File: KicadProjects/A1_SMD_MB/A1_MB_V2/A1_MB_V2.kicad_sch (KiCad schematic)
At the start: 0 parts

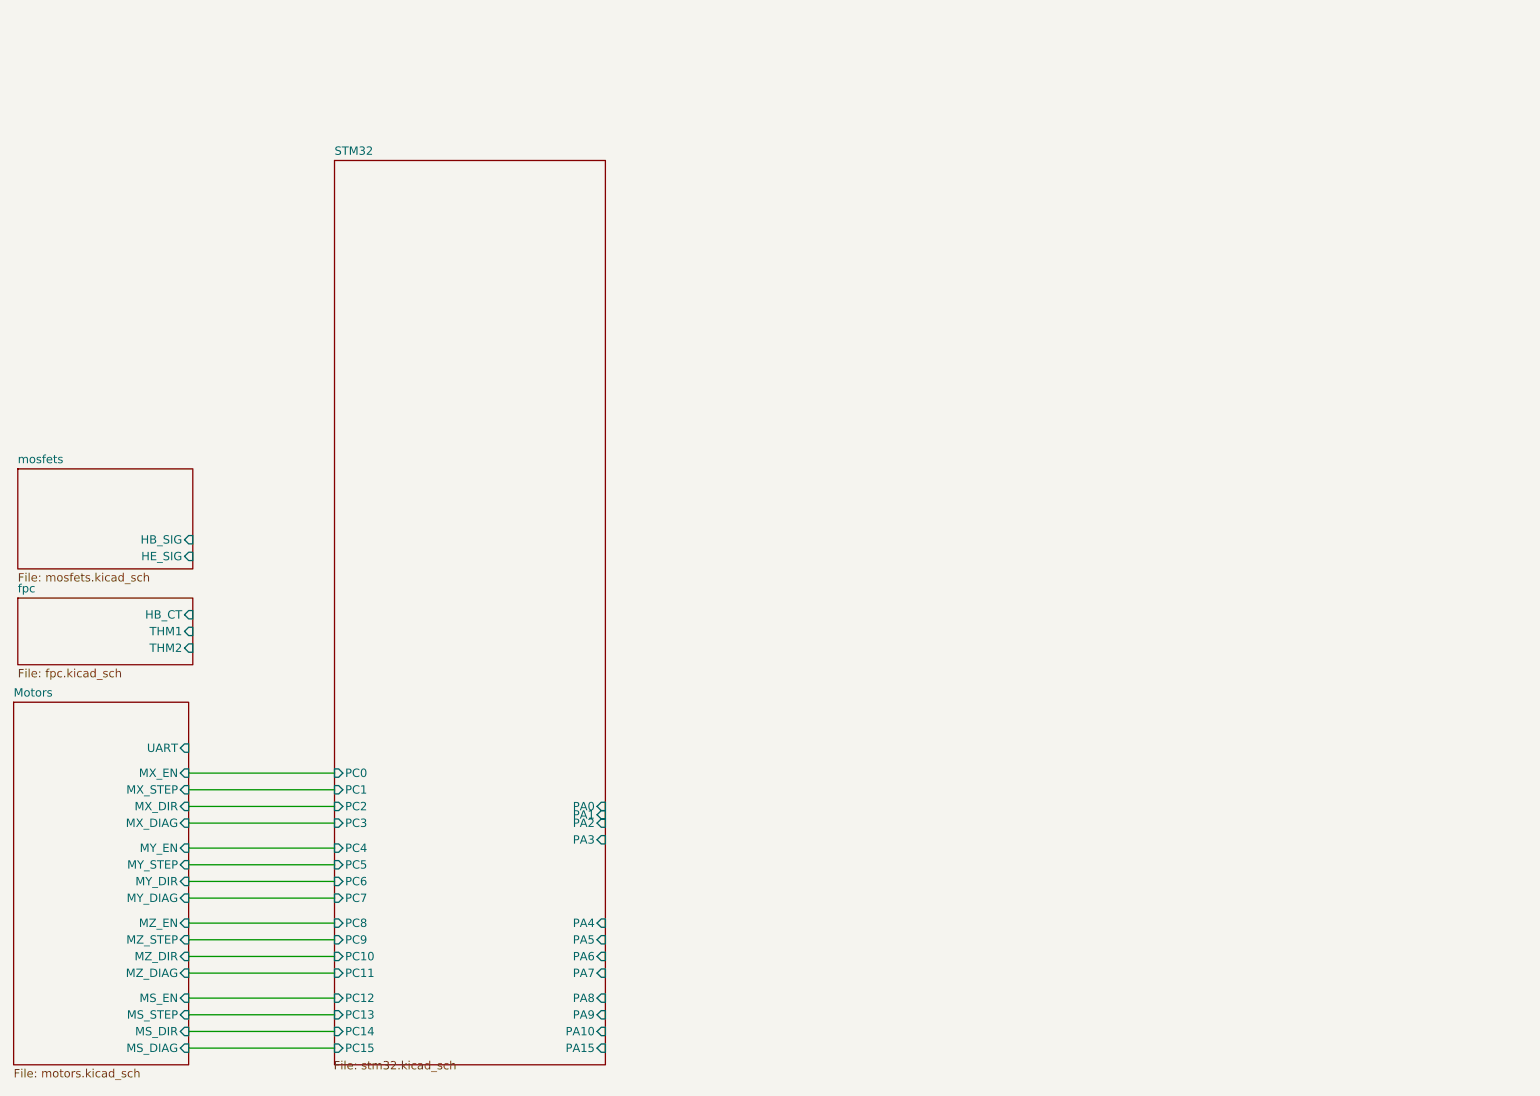
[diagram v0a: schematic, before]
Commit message: e
e
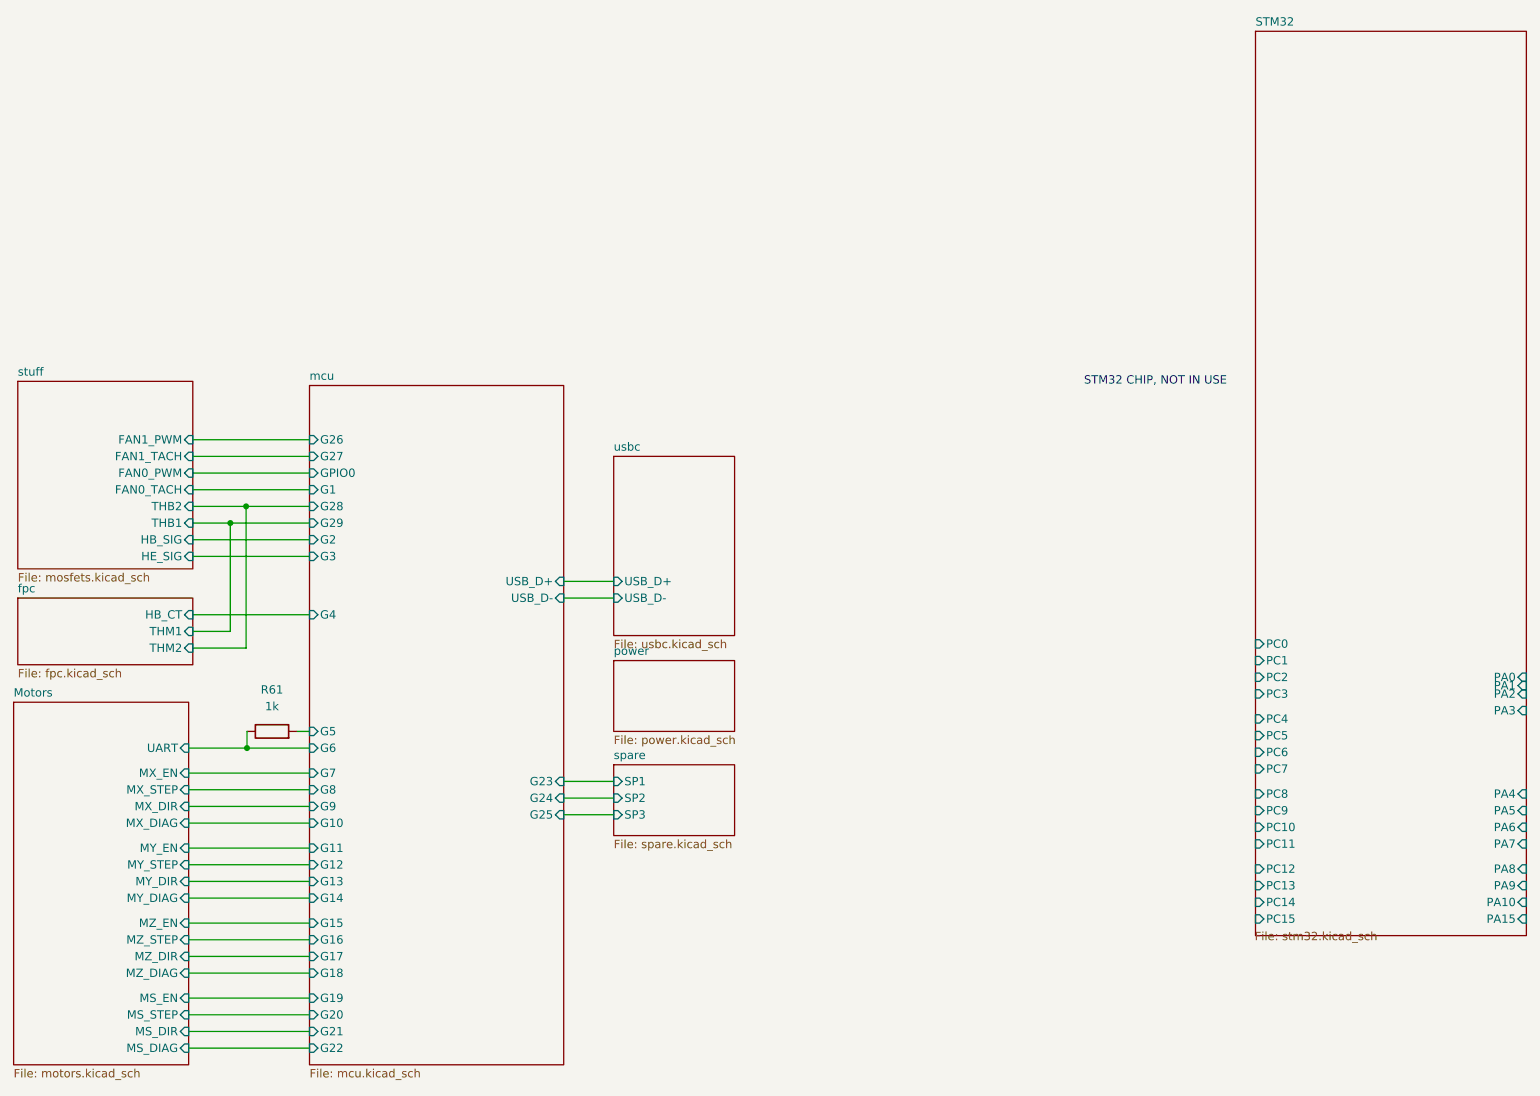
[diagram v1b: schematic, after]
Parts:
- added R61: 1k, symbol Device:R
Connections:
- net Motors/UART: now also R61.1
- new net mcu/G5: R61.2
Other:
- sheet mosfets renamed stuff
- added sheet mcu (mcu.kicad_sch)
- added sheet power (power.kicad_sch)
- added sheet spare (spare.kicad_sch)
- added sheet usbc (usbc.kicad_sch)
- sheet stuff ports: added FAN0_PWM, FAN0_TACH, FAN1_PWM, FAN1_TACH, THB1, THB2; removed none
- note added: "STM32 CHIP, NOT IN USE"
